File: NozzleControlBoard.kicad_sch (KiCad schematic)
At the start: 468 parts, among them IC2 MAX3094EESE+, IC3 MAX22245BAWA+, J1 24V_OUT, J101 SHIFT_DATA_TOSS, J102 8BIT_24V_IN, J103 SHIFT_DATA_TOSS, J104 8BIT_24V_OUT, J2 SHIFT_DATA_TOSS, J3 Conn_01x12_Male, J4 SHIFT_DATA_TOSS, J5 SHIFT_DATA_TOSS, J6 8BIT_24V_IN, J7 8BIT_24V_OUT, Q1 TPN22006NH,LQ, Q10 TPN22006NH,LQ, Q101 TPN22006NH,LQ, Q102 TPN22006NH,LQ, Q103 TPN22006NH,LQ, Q104 TPN22006NH,LQ, Q105 TPN22006NH,LQ, Q106 TPN22006NH,LQ, Q107 TPN22006NH,LQ, Q108 TPN22006NH,LQ, Q11 TPN22006NH,LQ, Q12 TPN22006NH,LQ, Q13 TPN22006NH,LQ, Q14 TPN22006NH,LQ, Q15 TPN22006NH,LQ, Q16 TPN22006NH,LQ, Q17 TPN22006NH,LQ, Q18 TPN22006NH,LQ, Q19 TPN22006NH,LQ, Q2 TPN22006NH,LQ, Q20 TPN22006NH,LQ, Q21 TPN22006NH,LQ, Q22 TPN22006NH,LQ, Q23 TPN22006NH,LQ, Q24 TPN22006NH,LQ, Q25 TPN22006NH,LQ, Q26 TPN22006NH,LQ, Q27 TPN22006NH,LQ, Q28 TPN22006NH,LQ, Q29 TPN22006NH,LQ, Q3 TPN22006NH,LQ, Q30 TPN22006NH,LQ, Q31 TPN22006NH,LQ, Q32 TPN22006NH,LQ, Q33 TPN22006NH,LQ, Q34 TPN22006NH,LQ, Q35 TPN22006NH,LQ, Q36 TPN22006NH,LQ, Q37 TPN22006NH,LQ, Q38 TPN22006NH,LQ, Q39 TPN22006NH,LQ, Q4 TPN22006NH,LQ, Q40 TPN22006NH,LQ, Q5 TPN22006NH,LQ, Q6 TPN22006NH,LQ, Q7 TPN22006NH,LQ, Q8 TPN22006NH,LQ, Q9 TPN22006NH,LQ, U1 74HCT595, U10 AP2127K-3.3, U101 74HC244, U102 74HCT595, U103 TLP291, U104 TLP291, U105 TLP291, U106 TLP291, U107 TLP291, U108 TLP291, U109 TLP291, U11 ATmega8A-A, U110 TLP291, U111 SOL9, U112 SOL10, U113 SOL11, U114 SOL12, U115 SOL13, U116 SOL14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

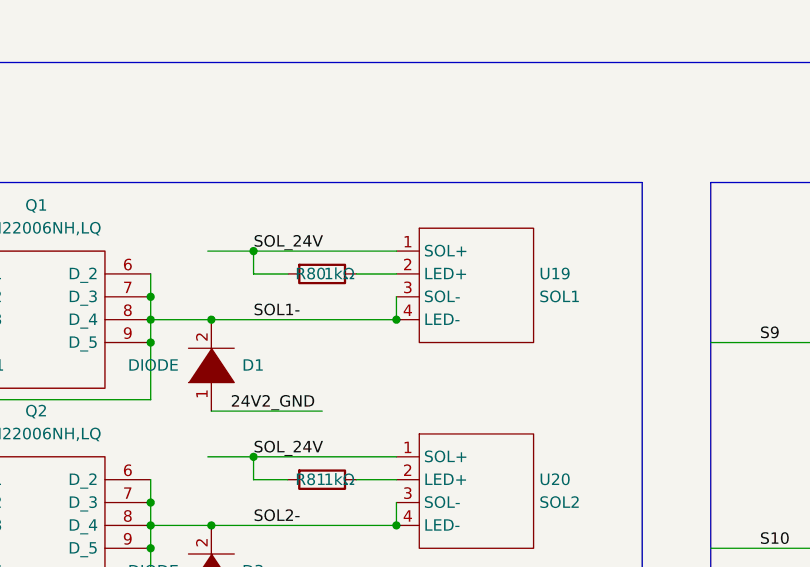
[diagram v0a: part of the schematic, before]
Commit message: .
.
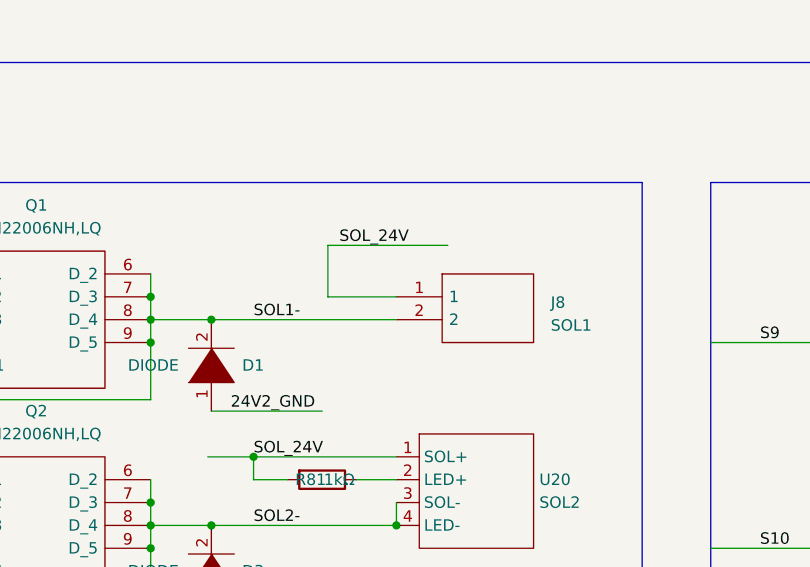
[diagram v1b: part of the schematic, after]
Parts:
- removed R80: 1kΩ, Resistor_SMD:R_0805_2012Metric, symbol Device:R
- removed U19: SOL1, SOL_PAD:SOL_PAD, symbol SOL_PAD_sym:SOL_PAD
- added J8: SOL1, footprint:2PIN, symbol 2pin:22-04-1021
- IC2: footprint MAX3094:SOIC127P600X175-16N -> footprint:SOIC127P600X175-16N
- IC3: footprint MAX22245:SOIC127P1031X265-8N -> footprint:SOIC127P1031X265-8N
- J1: footprint 24V_PAD:24V_PAD -> footprint:24V_PAD
- J103, J2: footprint SHIFT_DATA_TOSS:SHIFT_DATA_TOSS -> footprint:SHIFT_DATA_TOSS
- J3: footprint nozzle_input:input_pad -> footprint:input_pad
- PS1: footprint R05CTE05S:SOIC127P1030X265-16N -> footprint:SOIC127P1030X265-16N
- Q1: footprint TPN22006NH:TPN22006NHLQ -> footprint:TPN22006NHLQ
- U4: footprint ISP:4PIN_ISP -> footprint:4PIN_ISP
- U87: footprint sol_pad:sol_pad -> footprint:sol_pad
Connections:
- net 24V2: now also J8.1
- net SOL1-: now also J8.2
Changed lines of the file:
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@@
   (junction (at 1854.6926 272.4) (diameter 0) (color 0 0 0 0)
   )
-  (junction (at 784.86 125.095) (diameter 0) (color 0 0 0 0)
-  )
   (junction (at 2027.95 295.26) (diameter 0) (color 0 0 0 0)
   )
@@
   (junction (at 1875.255 158.1) (diameter 0) (color 0 0 0 0)
   )
-  (junction (at 800.735 132.715) (diameter 0) (color 0 0 0 0)
-  )
   (junction (at 773.43 224.155) (diameter 0) (color 0 0 0 0)
   )
@@
     (stroke (width 0) (type default))
   )
-  (wire (pts (xy 800.735 127.635) (xy 796.29 127.635))
-    (stroke (width 0) (type default))
-  )
   (wire (pts (xy 1257.3 243.84) (xy 1271.27 243.84))
     (stroke (width 0) (type default))
@@
     (stroke (width 0) (type default))
   )
+  (wire (pts (xy 800.735 130.175) (xy 793.115 130.175))
+    (stroke (width 0) (type default))
+  )
   (wire (pts (xy 1859.38 196.2) (xy 1875.255 196.2))
     (stroke (width 0) (type default))
@@
     (stroke (width 0) (type default))
   )
-  (wire (pts (xy 784.86 127.635) (xy 788.67 127.635))
-    (stroke (width 0) (type default))
-  )
   (polyline (pts (xy 1420 407.34) (xy 2170 407.34))
     (stroke (width 0) (type default))
@@
     (stroke (width 0) (type default))
   )
+  (wire (pts (xy 793.115 124.46) (xy 793.115 130.175))
+    (stroke (width 0) (type default))
+  )
   (wire (pts (xy 1822.55 231.76) (xy 1822.55 235.57))
     (stroke (width 0) (type default))
@@
     (stroke (width 0) (type default))
   )
-  (wire (pts (xy 779.78 125.095) (xy 784.86 125.095))
-    (stroke (width 0) (type default))
-  )
   (wire (pts (xy 1323.975 175.26) (xy 1319.53 175.26))
     (stroke (width 0) (type default))
@@
     (stroke (width 0) (type default))
   )
-  (wire (pts (xy 800.735 130.175) (xy 800.735 132.715))
-    (stroke (width 0) (type default))
-  )
   (wire (pts (xy 2000.01 274.94) (xy 2002.55 274.94))
     (stroke (width 0) (type default))
@@
     (stroke (width 0) (type default))
   )
-  (wire (pts (xy 784.86 127.635) (xy 784.86 125.095))
-    (stroke (width 0) (type default))
-  )
   (wire (pts (xy 1684.02 195.58) (xy 1699.895 195.58))
     (stroke (width 0) (type default))
@@
     (stroke (width 0) (type default))
   )
-  (wire (pts (xy 784.86 125.095) (xy 800.735 125.095))
-    (stroke (width 0) (type default))
-  )
   (wire (pts (xy 701.04 135.255) (xy 690.88 135.255))
     (stroke (width 0) (type default))
@@
     (stroke (width 0) (type default))
   )
+  (wire (pts (xy 793.115 124.46) (xy 806.45 124.46))
+    (stroke (width 0) (type default))
+  )
   (wire (pts (xy 406.4 93.98) (xy 425.45 93.98))
     (stroke (width 0) (type default))
@@
     (effects (font (size 1.27 1.27)) (justify left bottom))
   )
+  (label "SOL_24V" (at 794.385 124.46 0) (fields_autoplaced)
+    (effects (font (size 1.27 1.27)) (justify left bottom))
+  )
   (label "24V2_GND" (at 1991.12 221.6 0) (fields_autoplaced)
     (effects (font (size 1.27 1.27)) (justify left bottom))
@@
     (effects (font (size 1.27 1.27)) (justify left bottom))
   )
-  (label "SOL_24V" (at 784.86 125.095 0) (fields_autoplaced)
-    (effects (font (size 1.27 1.27)) (justify left bottom))
-  )
   (label "LATCH_3" (at 2139.7688 237.46 180) (fields_autoplaced)
     (effects (font (size 1.27 1.27)) (justify right bottom))
@@
       (effects (font (size 1.27 1.27)))
     )
-    (property "Footprint" "MAX3094:SOIC127P600X175-16N" (at 438.15 139.7 0)
+    (property "Footprint" "footprint:SOIC127P600X175-16N" (at 438.15 139.7 0)
       (effects (font (size 1.27 1.27)) (justify left) hide)
     )
@@
       (effects (font (size 1.27 1.27)))
     )
-    (property "Footprint" "ISP:4PIN_ISP" (at 518.16 325.12 0)
+    (property "Footprint" "footprint:4PIN_ISP" (at 518.16 325.12 0)
       (effects (font (size 1.27 1.27)) hide)
     )
@@
       (effects (font (size 1.27 1.27)))
     )
-    (property "Footprint" "R05CTE05S:SOIC127P1030X265-16N" (at 547.37 127 0)
+    (property "Footprint" "footprint:SOIC127P1030X265-16N" (at 547.37 127 0)
       (effects (font (size 1.27 1.27)) (justify left) hide)
     )
@@
       (effects (font (size 1.27 1.27)))
     )
-    (property "Footprint" "TPN22006NH:TPN22006NHLQ" (at 769.62 125.095 0)
+    (property "Footprint" "footprint:TPN22006NHLQ" (at 769.62 125.095 0)
       (effects (font (size 1.27 1.27)) (justify left) hide)
     )
@@
       (effects (font (size 1.27 1.27)) (justify left))
     )
-    (property "Footprint" "SHIFT_DATA_TOSS:SHIFT_DATA_TOSS" (at 2156.3745 240 0)
+    (property "Footprint" "footprint:SHIFT_DATA_TOSS" (at 2156.3745 240 0)
       (effects (font (size 1.27 1.27)) hide)
     )
@@
       (effects (font (size 1.27 1.27)))
     )
-    (property "Footprint" "MAX22245:SOIC127P1031X265-8N" (at 542.29 167.64 0)
+    (property "Footprint" "footprint:SOIC127P1031X265-8N" (at 542.29 167.64 0)
       (effects (font (size 1.27 1.27)) (justify left) hide)
     )
@@
       (effects (font (size 1.27 1.27)))
     )
-    (property "Footprint" "nozzle_input:input_pad" (at 401.32 101.6 0)
+    (property "Footprint" "footprint:input_pad" (at 401.32 101.6 0)
       (effects (font (size 1.27 1.27)) hide)
     )
@@
       (effects (font (size 1.27 1.27)) (justify left))
     )
-    (property "Footprint" "sol_pad:sol_pad" (at 2057.795 240.65 0)
+    (property "Footprint" "footprint:sol_pad" (at 2057.795 240.65 0)
       (effects (font (size 1.27 1.27)) hide)
     )
@@
       (effects (font (size 1.27 1.27)) (justify left))
     )
-    (property "Footprint" "SHIFT_DATA_TOSS:SHIFT_DATA_TOSS" (at 1028.7 228.6 0)
+    (property "Footprint" "footprint:SHIFT_DATA_TOSS" (at 1028.7 228.6 0)
       (effects (font (size 1.27 1.27)) hide)
     )
@@
     )
   )
+  (symbol (lib_id "2pin:22-04-1021") (at 800.735 130.175 0) (unit 1)
+    (in_bom yes) (on_board yes) (dnp no) (fields_autoplaced)
+    (property "Reference" "J8" (at 817.88 130.81 0)
+      (effects (font (size 1.27 1.27)) (justify left))
+    )
+    (property "Value" "SOL1" (at 817.88 133.35 0)
+      (effects (font (size 1.27 1.27)) (justify left))
+    )
+    (property "Footprint" "footprint:2PIN" (at 817.245 127.635 0)
+      (effects (font (size 1.27 1.27)) (justify left) hide)
+    )
+    (property "Datasheet" "https://componentsearchengine.com/Datasheets/2/22-04-1021.pdf" (at 817.245 130.175 0)
+      (effects (font (size 1.27 1.27)) (justify left) hide)
+    )
+    (property "Description" "Headers & Wire Housings 2P HEADER MINI-LATCH 2.5 HEADER ASS\\'Y ST WITH LOCK" (at 817.245 132.715 0)
+      (effects (font (size 1.27 1.27)) (justify left) hide)
+    )
+    (property "Height" "11.7" (at 817.245 135.255 0)
+      (effects (font (size 1.27 1.27)) (justify left) hide)
+    )
+    (property "Manufacturer_Name" "Molex" (at 817.245 137.795 0)
+      (effects (font (size 1.27 1.27)) (justify left) hide)
+    )
+    (property "Manufacturer_Part_Number" "22-04-1021" (at 817.245 140.335 0)
+      (effects (font (size 1.27 1.27)) (justify left) hide)
+    )
+    (property "Mouser Part Number" "538-22-04-1021" (at 817.245 142.875 0)
+      (effects (font (size 1.27 1.27)) (justify left) hide)
+    )
+    (property "Mouser Price/Stock" "https://www.mouser.co.uk/ProductDetail/Molex/22-04-1021?qs=EaMIwIL37xykdY82kJj2ug%3D%3D" (at 817.245 145.415 0)
+      (effects (font (size 1.27 1.27)) (justify left) hide)
+    )
+    (property "Arrow Part Number" "" (at 817.245 147.955 0)
+      (effects (font (size 1.27 1.27)) (justify left) hide)
+    )
+    (property "Arrow Price/Stock" "" (at 817.245 150.495 0)
+      (effects (font (size 1.27 1.27)) (justify left) hide)
+    )
+    (pin "1")
+    (pin "2")
+    (instances
+      (project "NozzleControlBoard"
+        (path "/c2c935bf-a0d6-42c1-aed8-051cbdf63e9b"
+          (reference "J8") (unit 1)
+        )
+      )
+    )
+  )
   (symbol (lib_id "74xx:74HC244") (at 1117.6 228.6 0) (unit 1)
     (in_bom yes) (on_board yes) (dnp no) (fields_autoplaced)
@@
     )
   )
-  (symbol (lib_id "SOL_PAD_sym:SOL_PAD") (at 803.275 122.555 0) (unit 1)
-    (in_bom yes) (on_board yes) (dnp no) (fields_autoplaced)
-    (property "Reference" "U19" (at 816.61 127.6349 0)
-      (effects (font (size 1.27 1.27)) (justify left))
-    )
-    (property "Value" "SOL1" (at 816.61 130.1749 0)
-      (effects (font (size 1.27 1.27)) (justify left))
-    )
-    (property "Footprint" "SOL_PAD:SOL_PAD" (at 803.275 123.825 0)
-      (effects (font (size 1.27 1.27)) hide)
-    )
-    (property "Datasheet" "" (at 803.275 123.825 0)
-      (effects (font (size 1.27 1.27)) hide)
-    )
-    (pin "1")
-    (pin "2")
-    (pin "3")
-    (pin "4")
-    (instances
-      (project "NozzleControlBoard"
-        (path "/c2c935bf-a0d6-42c1-aed8-051cbdf63e9b"
-          (reference "U19") (unit 1)
-        )
-      )
-    )
-  )
   (symbol (lib_id "Isolator:TLP291") (at 1963.18 226.68 0) (unit 1)
     (in_bom yes) (on_board yes) (dnp no) (fields_autoplaced)
@@
     )
   )
-  (symbol (lib_id "Device:R") (at 792.48 127.635 270) (unit 1)
-    (in_bom yes) (on_board yes) (dnp no)
-    (property "Reference" "R80" (at 791.21 127.635 90)
-      (effects (font (size 1.27 1.27)))
-    )
-    (property "Value" "1kΩ" (at 794.385 127.635 90)
-      (effects (font (size 1.27 1.27)))
-    )
-    (property "Footprint" "Resistor_SMD:R_0805_2012Metric" (at 792.48 125.857 90)
-      (effects (font (size 1.27 1.27)) hide)
-    )
-    (property "Datasheet" "~" (at 792.48 127.635 0)
-      (effects (font (size 1.27 1.27)) hide)
-    )
-    (pin "1")
-    (pin "2")
-    (instances
-      (project "NozzleControlBoard"
-        (path "/c2c935bf-a0d6-42c1-aed8-051cbdf63e9b"
-          (reference "R80") (unit 1)
-        )
-      )
-    )
-  )
   (symbol (lib_id "SOL_PAD_sym:SOL_PAD") (at 1326.515 215.9 0) (unit 1)
     (in_bom yes) (on_board yes) (dnp no) (fields_autoplaced)
@@
       (effects (font (size 1.27 1.27)))
     )
-    (property "Footprint" "24V_PAD:24V_PAD" (at 1029.97 256.54 0)
+    (property "Footprint" "footprint:24V_PAD" (at 1029.97 256.54 0)
       (effects (font (size 1.27 1.27)) hide)
     )

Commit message: .
.
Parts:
- removed R100, R101, R102, R103, R104, R81, R82, R83, R84, R85, R86, R87, R88, R89, R90, R91, R92, R93, R94, R95, R97, R98, R99: 1kΩ, Resistor_SMD:R_0805_2012Metric, symbol Device:R
- removed U20: SOL2, SOL_PAD:SOL_PAD, symbol SOL_PAD_sym:SOL_PAD
- removed U21: SOL3, SOL_PAD:SOL_PAD, symbol SOL_PAD_sym:SOL_PAD
- removed U22: SOL4, SOL_PAD:SOL_PAD, symbol SOL_PAD_sym:SOL_PAD
- removed U23: SOL5, SOL_PAD:SOL_PAD, symbol SOL_PAD_sym:SOL_PAD
- removed U24: SOL6, SOL_PAD:SOL_PAD, symbol SOL_PAD_sym:SOL_PAD
- removed U25: SOL7, SOL_PAD:SOL_PAD, symbol SOL_PAD_sym:SOL_PAD
- removed U26: SOL8, SOL_PAD:SOL_PAD, symbol SOL_PAD_sym:SOL_PAD
- removed U35: SOL9, SOL_PAD:SOL_PAD, symbol SOL_PAD_sym:SOL_PAD
- removed U36: SOL10, SOL_PAD:SOL_PAD, symbol SOL_PAD_sym:SOL_PAD
- removed U37: SOL11, SOL_PAD:SOL_PAD, symbol SOL_PAD_sym:SOL_PAD
- removed U38: SOL12, SOL_PAD:SOL_PAD, symbol SOL_PAD_sym:SOL_PAD
- removed U39: SOL13, SOL_PAD:SOL_PAD, symbol SOL_PAD_sym:SOL_PAD
- removed U40: SOL14, SOL_PAD:SOL_PAD, symbol SOL_PAD_sym:SOL_PAD
- removed U41: SOL15, SOL_PAD:SOL_PAD, symbol SOL_PAD_sym:SOL_PAD
- removed U42: SOL16, SOL_PAD:SOL_PAD, symbol SOL_PAD_sym:SOL_PAD
- removed U48: SOL9, sol_pad:sol_pad, symbol SOL_PAD_sym:SOL_PAD
- removed U49: SOL10, sol_pad:sol_pad, symbol SOL_PAD_sym:SOL_PAD
- removed U50: SOL11, sol_pad:sol_pad, symbol SOL_PAD_sym:SOL_PAD
- removed U51: SOL12, sol_pad:sol_pad, symbol SOL_PAD_sym:SOL_PAD
- removed U52: SOL13, sol_pad:sol_pad, symbol SOL_PAD_sym:SOL_PAD
- removed U53: SOL14, sol_pad:sol_pad, symbol SOL_PAD_sym:SOL_PAD
- removed U54: SOL15, sol_pad:sol_pad, symbol SOL_PAD_sym:SOL_PAD
- removed U55: SOL16, sol_pad:sol_pad, symbol SOL_PAD_sym:SOL_PAD
- added J10: SOL3, footprint:2PIN, symbol 2pin:22-04-1021
- added J11: SOL4, footprint:2PIN, symbol 2pin:22-04-1021
- added J12: SOL5, footprint:2PIN, symbol 2pin:22-04-1021
- added J13: SOL6, footprint:2PIN, symbol 2pin:22-04-1021
- added J14: SOL7, footprint:2PIN, symbol 2pin:22-04-1021
- added J15: SOL8, footprint:2PIN, symbol 2pin:22-04-1021
- added J16: SOL9, footprint:2PIN, symbol 2pin:22-04-1021
- added J17: SOL10, footprint:2PIN, symbol 2pin:22-04-1021
- added J18: SOL11, footprint:2PIN, symbol 2pin:22-04-1021
- added J19: SOL12, footprint:2PIN, symbol 2pin:22-04-1021
- added J20: SOL13, footprint:2PIN, symbol 2pin:22-04-1021
- added J21: SOL14, footprint:2PIN, symbol 2pin:22-04-1021
- added J22: SOL15, footprint:2PIN, symbol 2pin:22-04-1021
- added J23: SOL16, footprint:2PIN, symbol 2pin:22-04-1021
- added J24: SOL17, footprint:2PIN, symbol 2pin:22-04-1021
- added J25: SOL18, footprint:2PIN, symbol 2pin:22-04-1021
- added J26: SOL19, footprint:2PIN, symbol 2pin:22-04-1021
- added J27: SOL20, footprint:2PIN, symbol 2pin:22-04-1021
- added J28: SOL21, footprint:2PIN, symbol 2pin:22-04-1021
- added J29: SOL22, footprint:2PIN, symbol 2pin:22-04-1021
- added J30: SOL23, footprint:2PIN, symbol 2pin:22-04-1021
- added J31: SOL24, footprint:2PIN, symbol 2pin:22-04-1021
- added J9: SOL2, footprint:2PIN, symbol 2pin:22-04-1021
- Q10, Q11, Q12, Q13, Q14, Q15, Q16, Q17, Q18, Q19, Q2, Q20, Q21, Q22, Q23, Q24, Q3, Q5, Q6, Q7, Q8, Q9: footprint TPN22006NH:TPN22006NHLQ -> footprint:TPN22006NHLQ
- U5: footprint 74HCT244:SOP65P640X110-20N -> footprint:SOP65P640X110-20N
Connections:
- net 24V2: now also J10.1, J11.1, J12.1, J13.1, J14.1, J15.1, J16.1, J17.1, J18.1, J19.1, J20.1, J21.1, J22.1, J23.1, J24.1, J25.1, J26.1, J27.1, J28.1, J29.1, J30.1, J31.1, J9.1
- net SOL10-: now also J17.2
- net SOL11-: now also J18.2
- net SOL12-: now also J19.2
- net SOL13-: now also J20.2
- net SOL14-: now also J21.2
- net SOL15-: now also J22.2
- net SOL16-: now also J23.2
- net SOL17-: now also J24.2
- net SOL18-: now also J25.2
- net SOL19-: now also J26.2
- net SOL2-: now also J9.2
- net SOL20-: now also J27.2
- net SOL21-: now also J28.2
- net SOL22-: now also J29.2
- net SOL23-: now also J30.2
- net SOL24-: now also J31.2
- net SOL3-: now also J10.2
- net SOL4-: now also J11.2
- net SOL5-: now also J12.2
- net SOL6-: now also J13.2
- net SOL7-: now also J14.2
- net SOL8-: now also J15.2
- net SOL9-: now also J16.2

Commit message: ,
,
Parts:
- removed R130, R131, R132, R133, R134, R135, R136, R137, R162, R163, R164, R165, R166, R167, R168, R169, R194, R195, R196, R197, R198, R199, R200, R201: 1kΩ, Resistor_SMD:R_0805_2012Metric, symbol Device:R
- removed U111, U65, U82: SOL9, sol_pad:sol_pad, symbol SOL_PAD_sym:SOL_PAD
- removed U112, U66, U83: SOL10, sol_pad:sol_pad, symbol SOL_PAD_sym:SOL_PAD
- removed U113, U67, U84: SOL11, sol_pad:sol_pad, symbol SOL_PAD_sym:SOL_PAD
- removed U114, U68, U85: SOL12, sol_pad:sol_pad, symbol SOL_PAD_sym:SOL_PAD
- removed U115, U69, U86: SOL13, sol_pad:sol_pad, symbol SOL_PAD_sym:SOL_PAD
- removed U116, U70: SOL14, sol_pad:sol_pad, symbol SOL_PAD_sym:SOL_PAD
- removed U117, U71, U88: SOL15, sol_pad:sol_pad, symbol SOL_PAD_sym:SOL_PAD
- removed U118, U72, U89: SOL16, sol_pad:sol_pad, symbol SOL_PAD_sym:SOL_PAD
- removed U87: SOL14, footprint:sol_pad, symbol SOL_PAD_sym:SOL_PAD
- added J32: SOL25, footprint:2PIN, symbol 2pin:22-04-1021
- added J33: SOL26, footprint:2PIN, symbol 2pin:22-04-1021
- added J34: SOL27, footprint:2PIN, symbol 2pin:22-04-1021
- added J35: SOL28, footprint:2PIN, symbol 2pin:22-04-1021
- added J36: SOL29, footprint:2PIN, symbol 2pin:22-04-1021
- added J37: SOL30, footprint:2PIN, symbol 2pin:22-04-1021
- added J38: SOL31, footprint:2PIN, symbol 2pin:22-04-1021
- added J39: SOL32, footprint:2PIN, symbol 2pin:22-04-1021
- added J40: SOL33, footprint:2PIN, symbol 2pin:22-04-1021
- added J41: SOL34, footprint:2PIN, symbol 2pin:22-04-1021
- added J42: SOL35, footprint:2PIN, symbol 2pin:22-04-1021
- added J43: SOL36, footprint:2PIN, symbol 2pin:22-04-1021
- added J44: SOL37, footprint:2PIN, symbol 2pin:22-04-1021
- added J45: SOL38, footprint:2PIN, symbol 2pin:22-04-1021
- added J46: SOL39, footprint:2PIN, symbol 2pin:22-04-1021
- added J47: SOL40, footprint:2PIN, symbol 2pin:22-04-1021
- added J48: SOL41, footprint:2PIN, symbol 2pin:22-04-1021
- added J49: SOL42, footprint:2PIN, symbol 2pin:22-04-1021
- added J50: SOL43, footprint:2PIN, symbol 2pin:22-04-1021
- added J51: SOL44, footprint:2PIN, symbol 2pin:22-04-1021
- added J52: SOL45, footprint:2PIN, symbol 2pin:22-04-1021
- added J53: SOL46, footprint:2PIN, symbol 2pin:22-04-1021
- added J54: SOL47, footprint:2PIN, symbol 2pin:22-04-1021
- added J55: SOL48, footprint:2PIN, symbol 2pin:22-04-1021
- Q101, Q102, Q103, Q104, Q105, Q106, Q107, Q108, Q25, Q26, Q27, Q28, Q29, Q30, Q31, Q32, Q33, Q34, Q35, Q36, Q37, Q38, Q39, Q40: footprint TPN22006NH:TPN22006NHLQ -> footprint:TPN22006NHLQ
- U101: footprint 74HCT244:SOP65P640X110-20N -> footprint:SOP65P640X110-20N
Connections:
- net 24V2: now also J32.1, J33.1, J34.1, J35.1, J36.1, J37.1, J38.1, J39.1, J40.1, J41.1, J42.1, J43.1, J44.1, J45.1, J46.1, J47.1, J48.1, J49.1, J50.1, J51.1, J52.1, J53.1, J54.1, J55.1
- net SOL25-: now also J32.2
- net SOL26-: now also J33.2
- net SOL27-: now also J34.2
- net SOL28-: now also J35.2
- net SOL29-: now also J36.2
- net SOL30-: now also J37.2
- net SOL31-: now also J38.2
- net SOL32-: now also J39.2
- net SOL33-: now also J40.2
- net SOL34-: now also J41.2
- net SOL35-: now also J42.2
- net SOL36-: now also J43.2
- net SOL37-: now also J44.2
- net SOL38-: now also J45.2
- net SOL39-: now also J46.2
- net SOL40-: now also J47.2
- net SOL41-: now also J48.2
- net SOL42-: now also J49.2
- net SOL43-: now also J50.2
- net SOL44-: now also J51.2
- net SOL45-: now also J52.2
- net SOL46-: now also J53.2
- net SOL47-: now also J54.2
- net SOL48-: now also J55.2
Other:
- moved on the sheet: J1, J2
